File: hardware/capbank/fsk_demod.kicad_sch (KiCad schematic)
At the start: 25 parts, among them U10 TS861IL, U17 MCP4012-xxxxCH, U6 MCP6021T-E-OT, U7 74HC4046AD

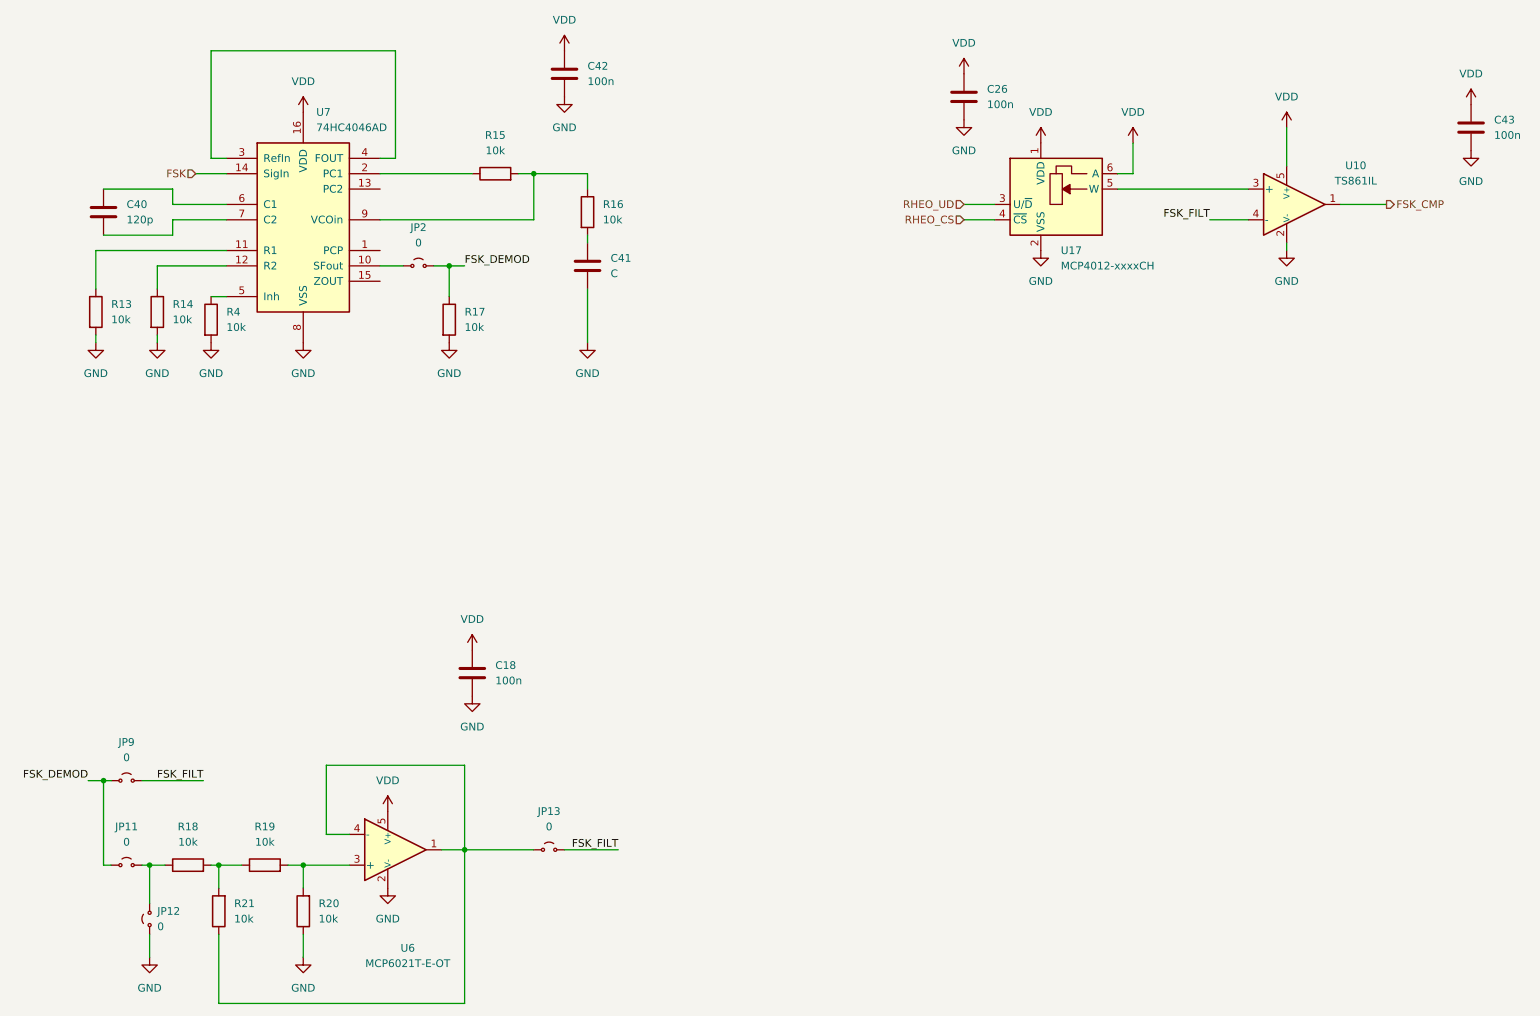
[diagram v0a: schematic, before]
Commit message: Update PCB with learned lessons
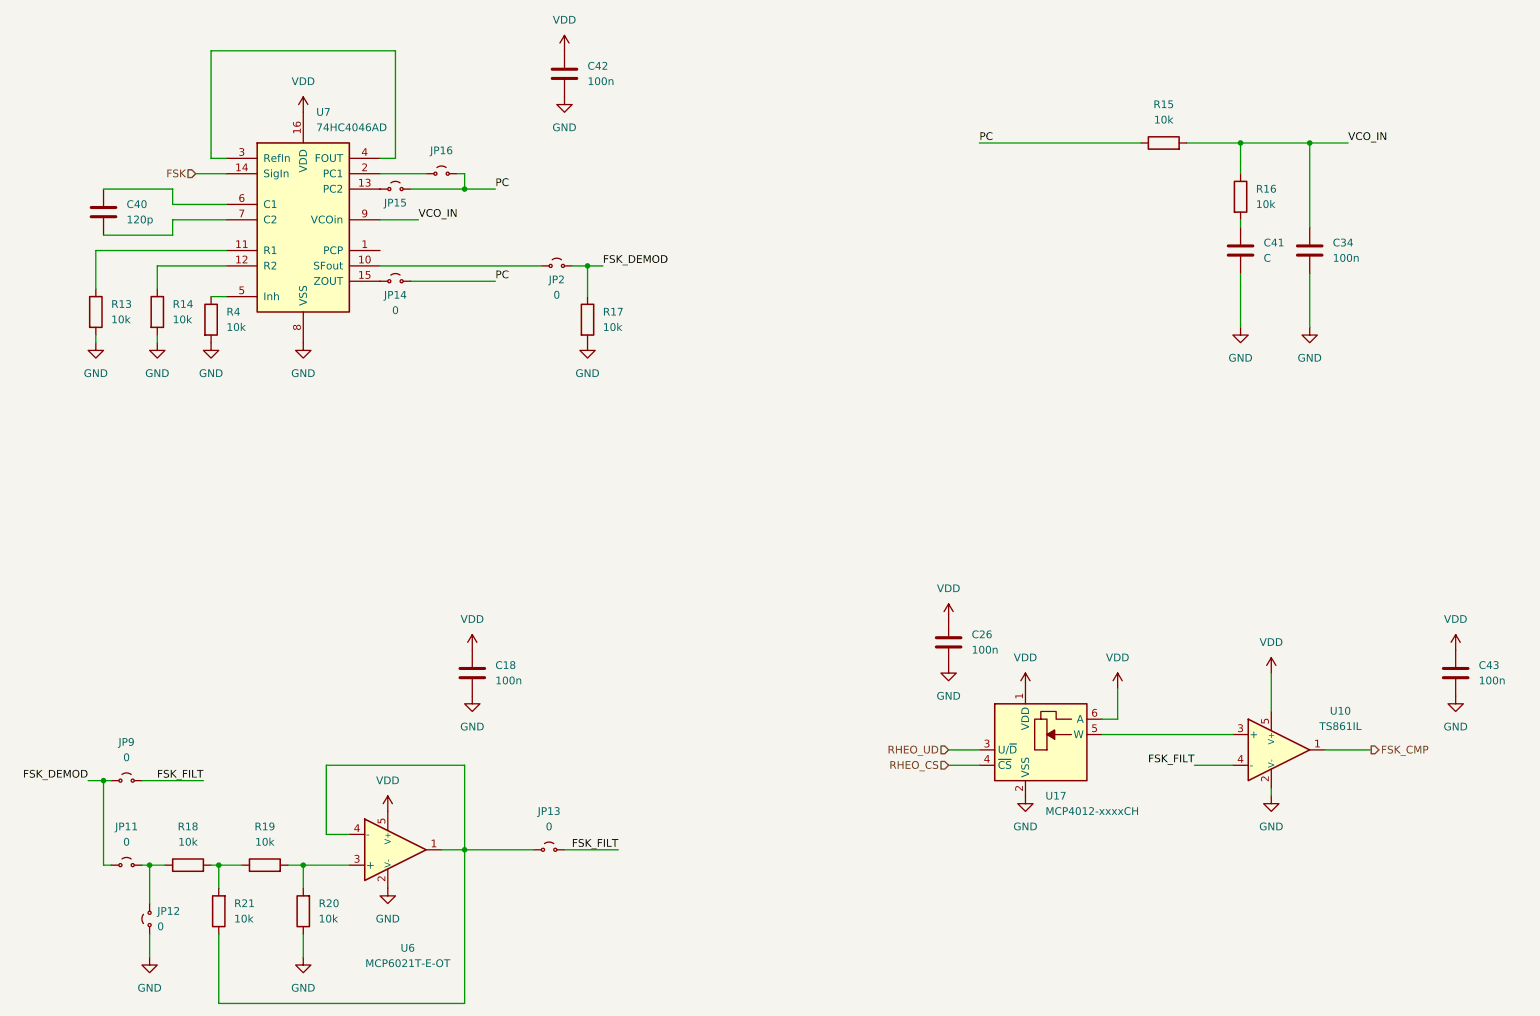
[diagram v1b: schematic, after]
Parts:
- added C34: 100n, PCM_Capacitor_SMD_AKL:C_0603_1608Metric, symbol Device:C
- added JP14, JP15, JP16: 0, PCM_Resistor_SMD_AKL:R_0603_1608Metric, symbol Jumper:Jumper_2_Small_Open
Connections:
- net GND: now also C34.2
- net VCO_IN: now reaches R15.2, R16.1, U7.9 (VCOin)
- net VCO_IN: now also C34.1
- net at U7.2 (PC1): now also JP16.1 (A); no longer R15.1
- net at U7.13 (PC2): now also JP15.1 (A)
- net at U7.15 (ZOUT): now also JP14.1 (A)
- new net PC: JP14.2 (B), JP15.2 (B), JP16.2 (B), R15.1
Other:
- moved on the sheet: C26, C41, C43, JP2, R15, R16, R17, U10, U17
